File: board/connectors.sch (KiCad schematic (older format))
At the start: 16 parts, among them J2 Conn_ARM_JTAG_SWD_10, J3 USB_B_Micro, J4 Conn_01x04_Male, J5 Screw_Terminal_01x02, U6 USBLC6-2SC6

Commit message: Update
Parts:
- J3: footprint Connector_USB:USB_Micro-B_Amphenol_10103594-0001LF_Horizontal -> Connector_USB:USB_Micro-B_Molex_47346-0001
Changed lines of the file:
@@
 F 0 "J3" H 4057 2767 50  0000 C CNN
 F 1 "USB_B_Micro" H 4057 2676 50  0000 C CNN
-F 2 "Connector_USB:USB_Micro-B_Amphenol_10103594-0001LF_Horizontal" H 4150 2250 50  0001 C CNN
+F 2 "Connector_USB:USB_Micro-B_Molex_47346-0001" H 4150 2250 50  0001 C CNN
 F 3 "~" H 4150 2250 50  0001 C CNN
 	1    4000 2300

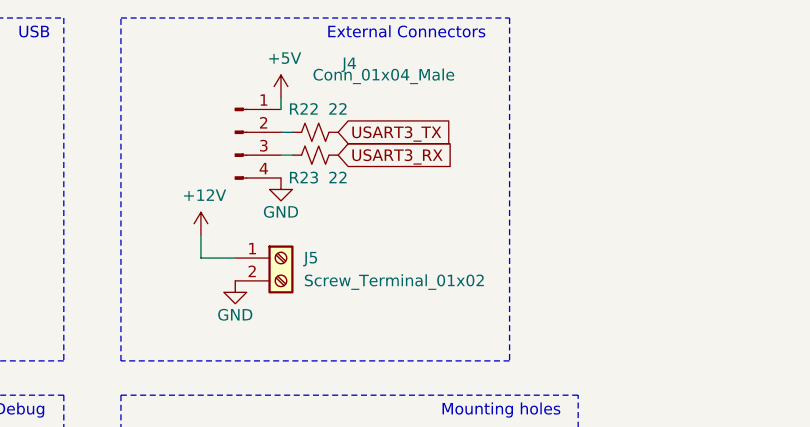
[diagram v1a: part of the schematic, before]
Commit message: ok
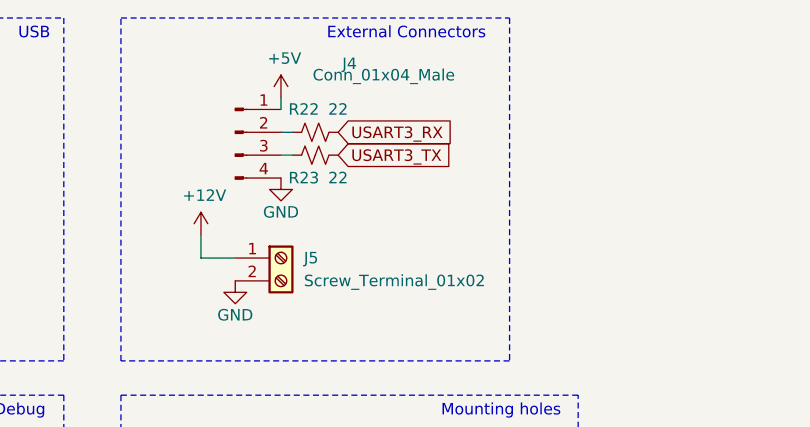
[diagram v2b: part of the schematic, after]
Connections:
- net USART3_RX: now also R22.1; no longer R23.1
- net USART3_TX: now also R23.1; no longer R22.1
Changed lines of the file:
@@
 Text Notes 4500 3250 0    50   ~ 0
 Serial Wire Debug\n
+Text GLabel 6400 2100 2    50   Input ~ 0
+USART3_TX
 Text GLabel 6400 2000 2    50   Input ~ 0
-USART3_TX
-Text GLabel 6400 2100 2    50   Input ~ 0
 USART3_RX
 $Comp
